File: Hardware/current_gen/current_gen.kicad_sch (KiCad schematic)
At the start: 28 parts, among them J1 Conn_Coaxial, J2 Conn_Coaxial, J3 Jack-DC, J4 Conn_Coaxial, Q1 NPN, Q10 NPN, Q11 NPN, Q12 NPN, Q13 BSP129, Q2 NPN, Q3 NPN, Q4 NPN, Q5 NPN, Q6 NPN, Q7 NPN, Q8 NPN, Q9 NPN, U1 OPA2673

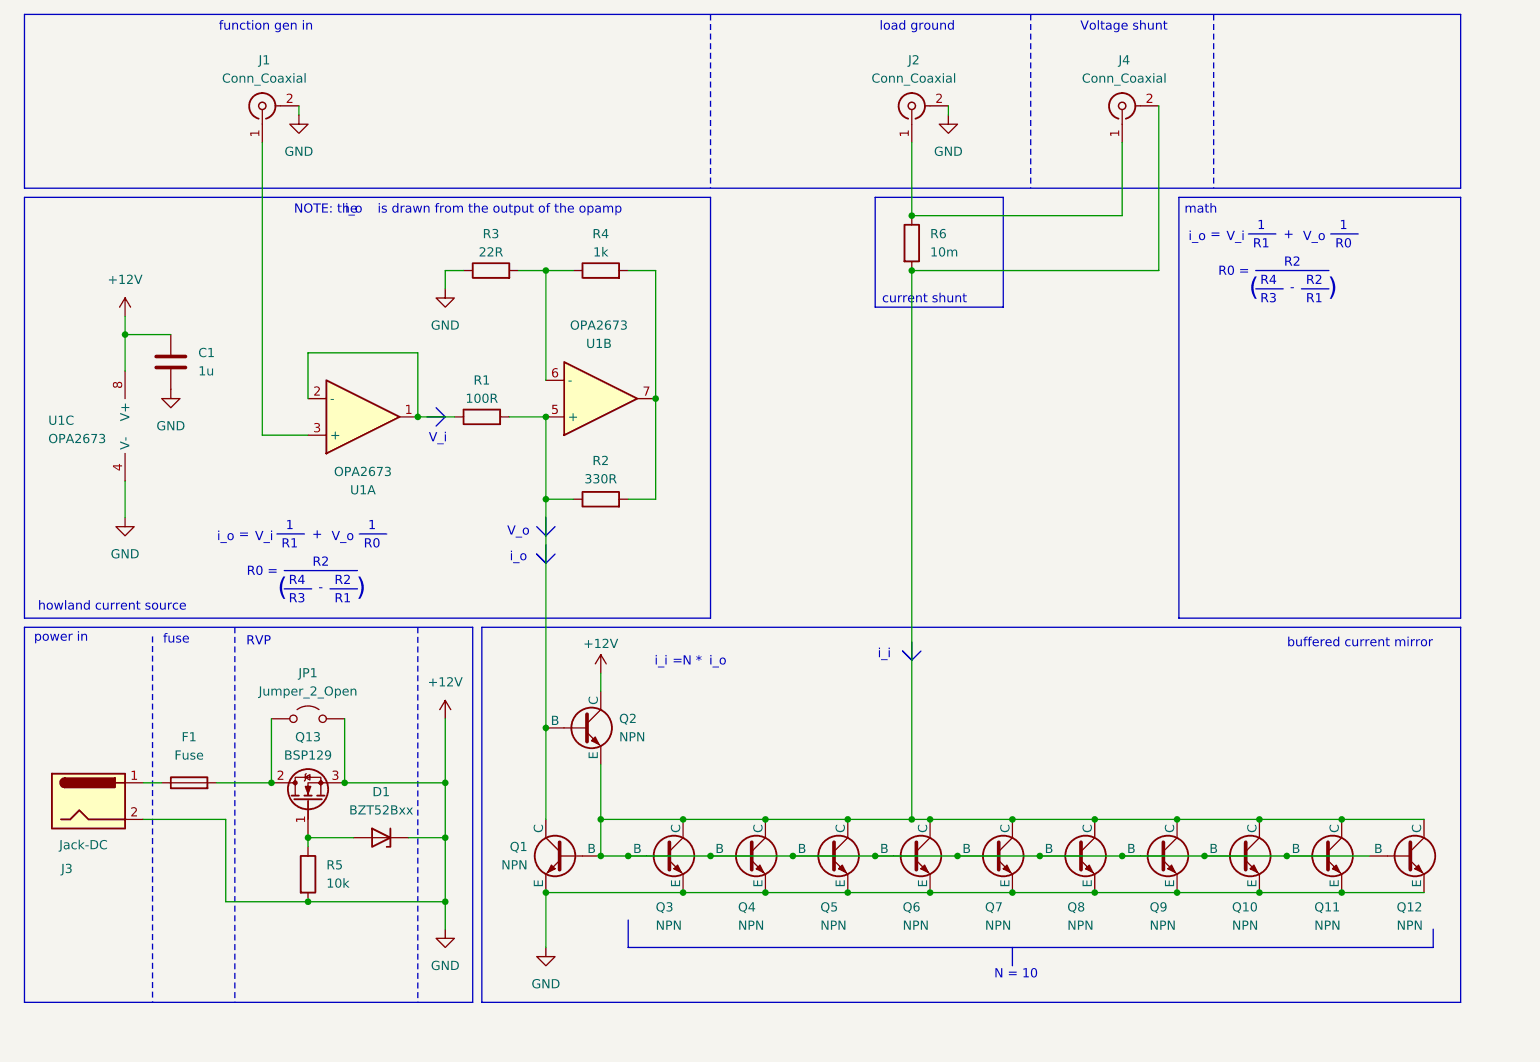
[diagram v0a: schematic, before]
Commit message: added some docs
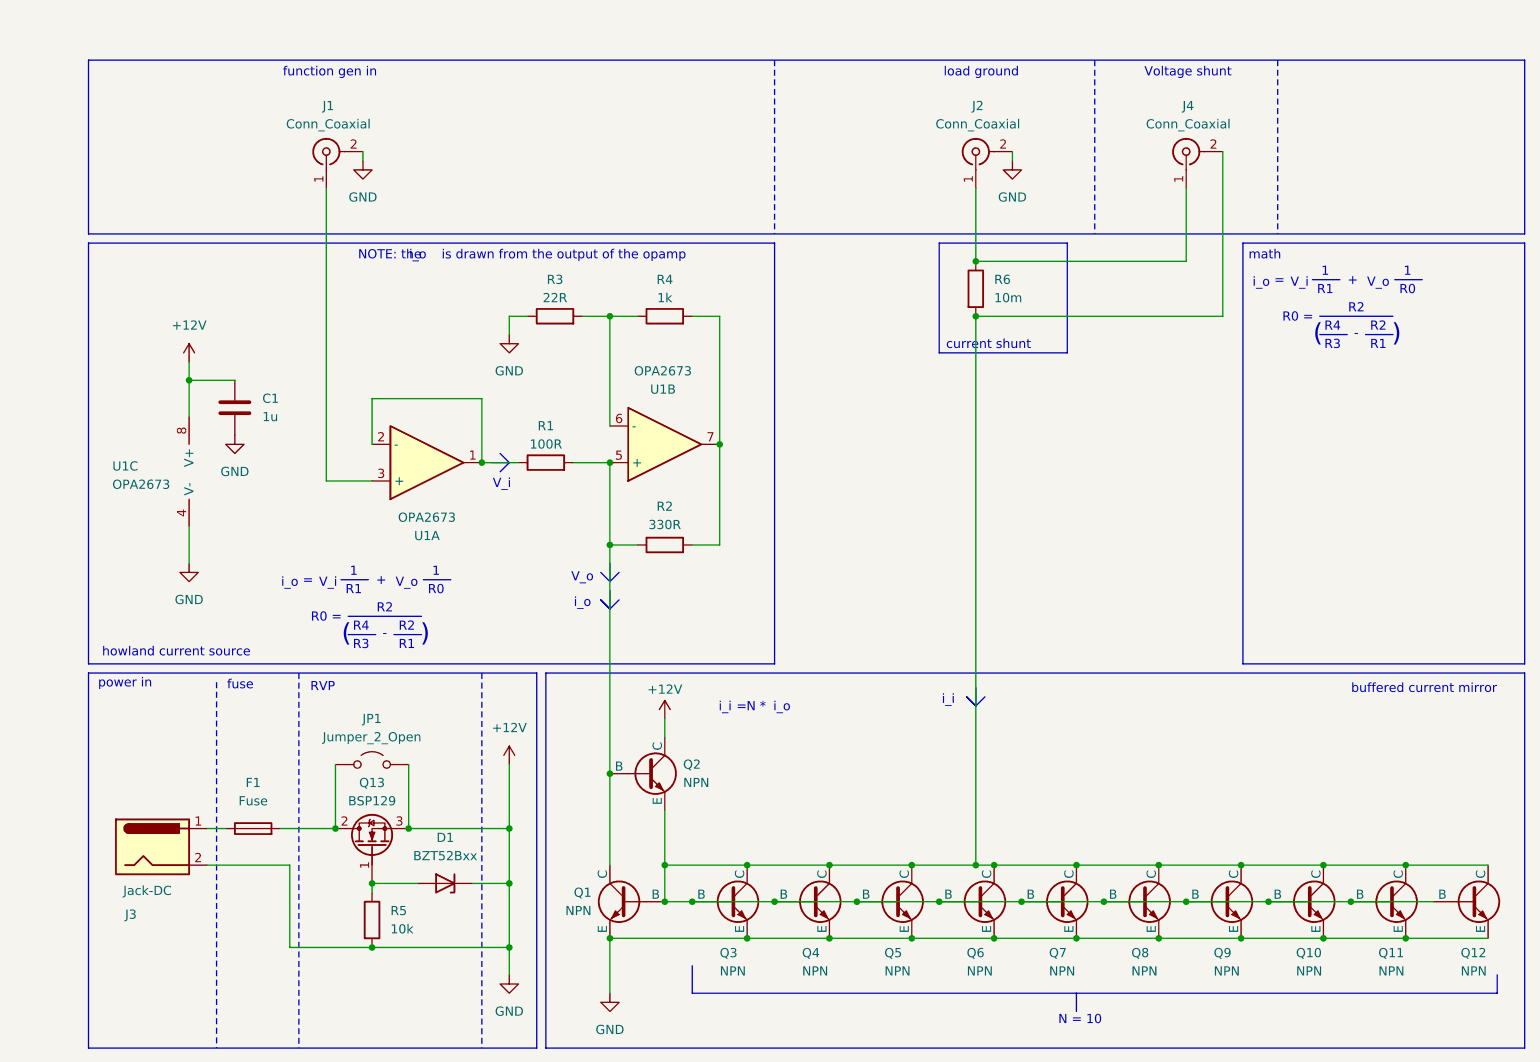
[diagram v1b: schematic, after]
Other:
- title: (none) -> constant current function gen
- moved on the sheet: C1, D1, F1, J1, J2, J3, J4, JP1, Q1, Q10, Q11, Q12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
